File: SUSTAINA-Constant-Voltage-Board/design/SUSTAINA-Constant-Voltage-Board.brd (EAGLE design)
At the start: 67 x 82 mm, 51 parts, among them M1 I7C4W012A050V-0C1-R, M2 POWER-MONITOR-MODULE, M3 USB-TO-QUAD-RS-485-CONV-MODUL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

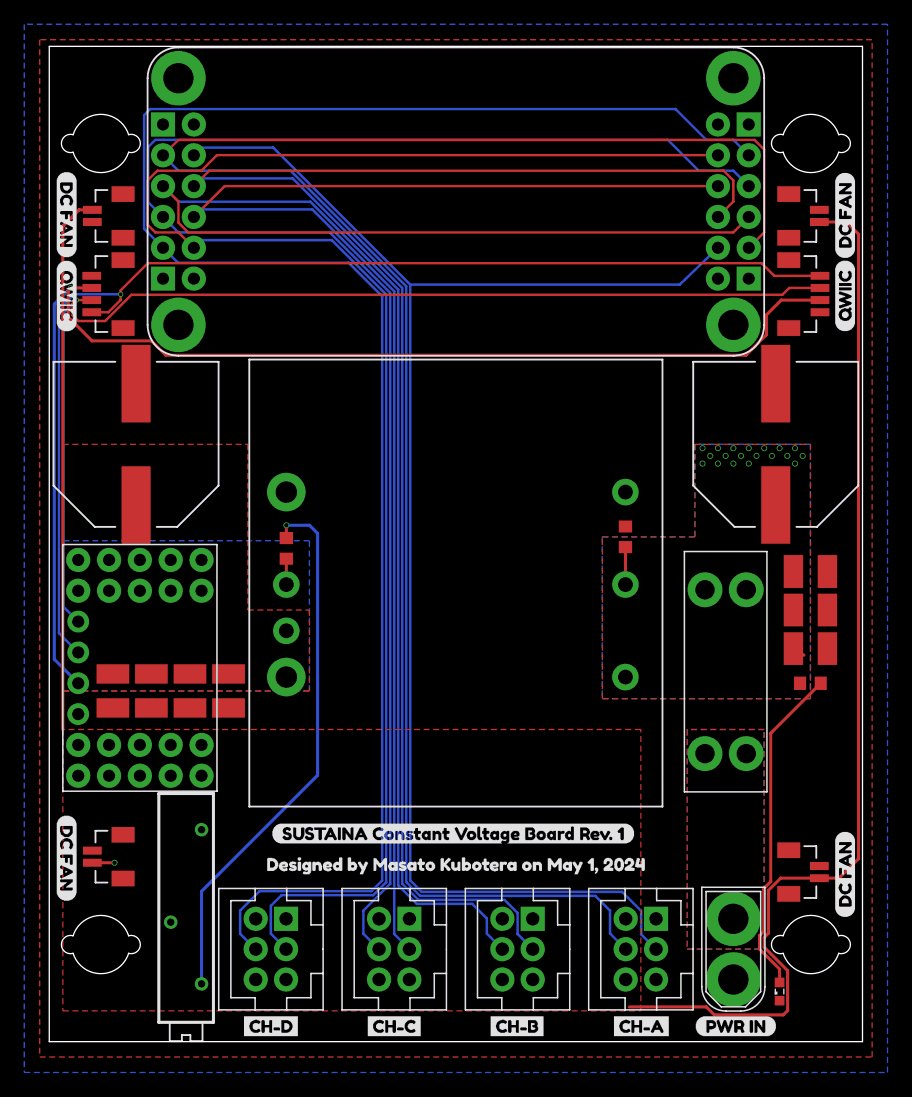
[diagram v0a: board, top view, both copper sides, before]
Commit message: Revert Constant-Voltage-Board to version without fan connectors and add data and documentation for outsourcing
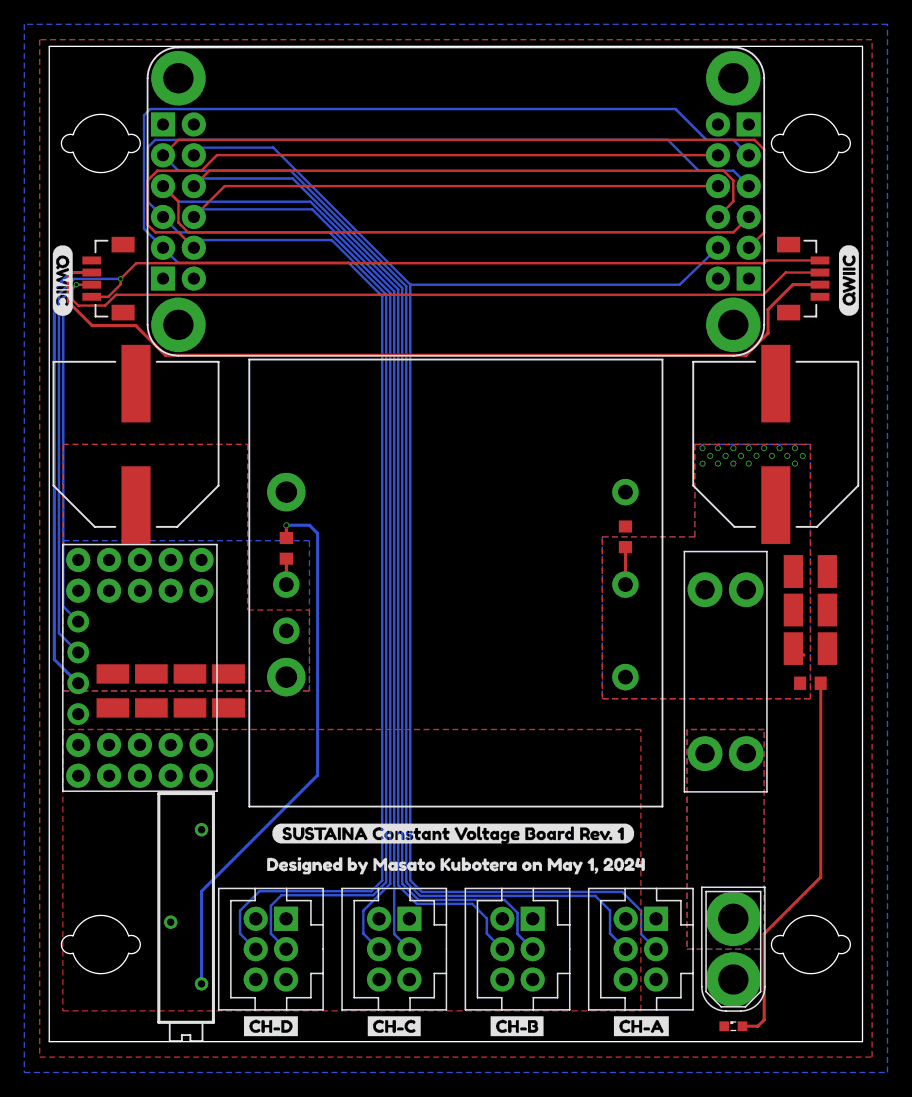
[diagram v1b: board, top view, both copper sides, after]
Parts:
- removed CH10, CH11, CH8, CH9: BM02B-SRSS-TB, SH-Connecters:BM02B-SRSS-TB
- removed U$19, U$20, U$21, U$22: (no value), buzzard_labels:DC_FAN
- removed U$5: (no value), buzzard_labels:PWR_IN0
- moved LED1 4.76 mm to (22.9, 1.27), turned to 0 degrees
- moved U$6 1.31 mm to (32.4, 59.7)
- moved U$7 1.31 mm to (-32.4, 65.7)
- moved CH6 1.27 mm to (26.7, 62.9)
- moved CH7 1.27 mm to (-26.7, 62.9)
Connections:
- net GND: no longer CH10.1, CH11.1, CH8.1, CH9.1
- net PWR_OUT: no longer CH10.2, CH11.2, CH8.2, CH9.2
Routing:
- net PWR_OUT: track 132.4 -> 0.00 mm
- net LED_DCDC-IN: track 27.4 -> 31.7 mm
- net +3V3: track 104.2 -> 106.7 mm
- net GND: track 1.87 -> 0.00 mm, vias 1 -> 0
- net SDA: track 93.0 -> 94.3 mm

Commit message: Added connector for DC fans to SUSTAINA-Constant-Voltage-Board
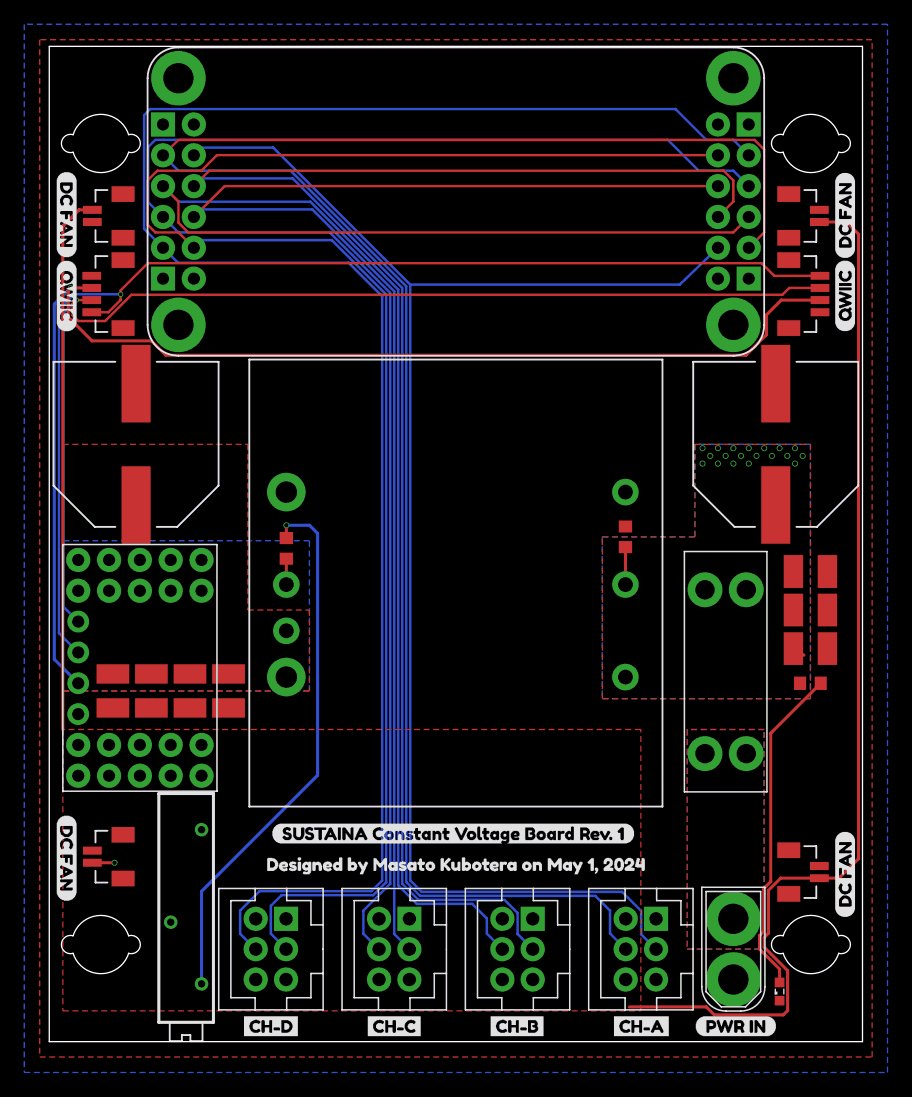
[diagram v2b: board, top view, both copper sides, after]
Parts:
- added CH10, CH11, CH8, CH9: BM02B-SRSS-TB, SH-Connecters:BM02B-SRSS-TB
- added U$19, U$20, U$21, U$22: (no value), buzzard_labels:DC_FAN
- added U$5: (no value), buzzard_labels:PWR_IN0
- moved LED1 4.76 mm to (26.7, 4.13), turned to 90 degrees
- moved U$6 1.31 mm to (32.1, 58.4)
- moved U$7 1.31 mm to (-32.1, 64.5)
- moved CH6 1.27 mm to (26.7, 61.6)
- moved CH7 1.27 mm to (-26.7, 61.6)
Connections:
- net GND: now also CH10.1, CH11.1, CH8.1, CH9.1
- net PWR_OUT: now also CH10.2, CH11.2, CH8.2, CH9.2
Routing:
- net PWR_OUT: track 0.00 -> 132.4 mm
- net LED_DCDC-IN: track 31.7 -> 27.4 mm
- net +3V3: track 106.7 -> 104.2 mm
- net GND: track 0.00 -> 1.87 mm, vias 0 -> 1
- net SDA: track 94.3 -> 93.0 mm
